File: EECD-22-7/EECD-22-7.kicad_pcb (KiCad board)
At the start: 2 copper layers, 55 parts, among them J1 Screw_Terminal_01x03, J2 Screw_Terminal_01x04, J3 Screw_Terminal_01x02, J4 Conn_ARM_JTAG_SWD_10, J5 Screw_Terminal_01x02, Q1 IRF6616, Q2 IRF6616, SW1 SW_Push, U1 4002B, U10 STM32F103CBUx, U7 LMR54406DBVR, U8 LMR54406DBVR, U9 LMR54406DBVR

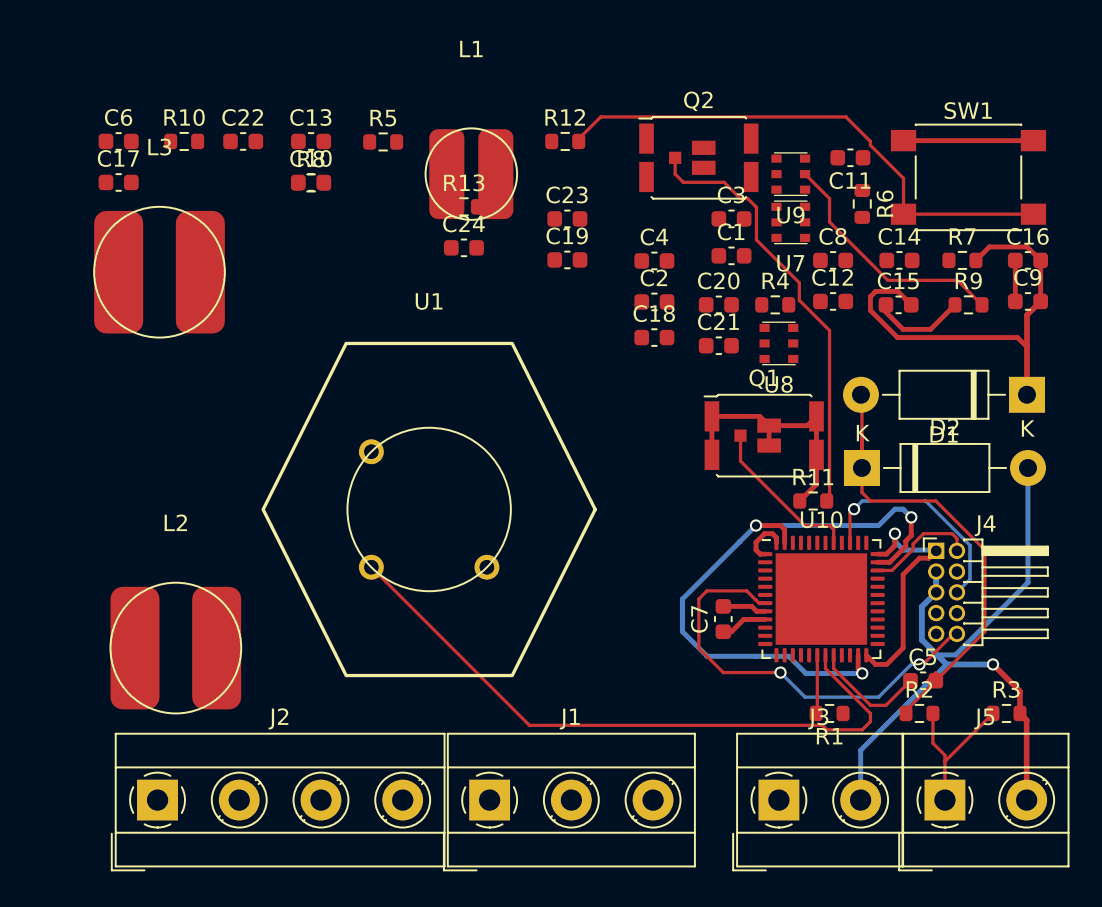
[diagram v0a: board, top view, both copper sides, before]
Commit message: Add files via upload
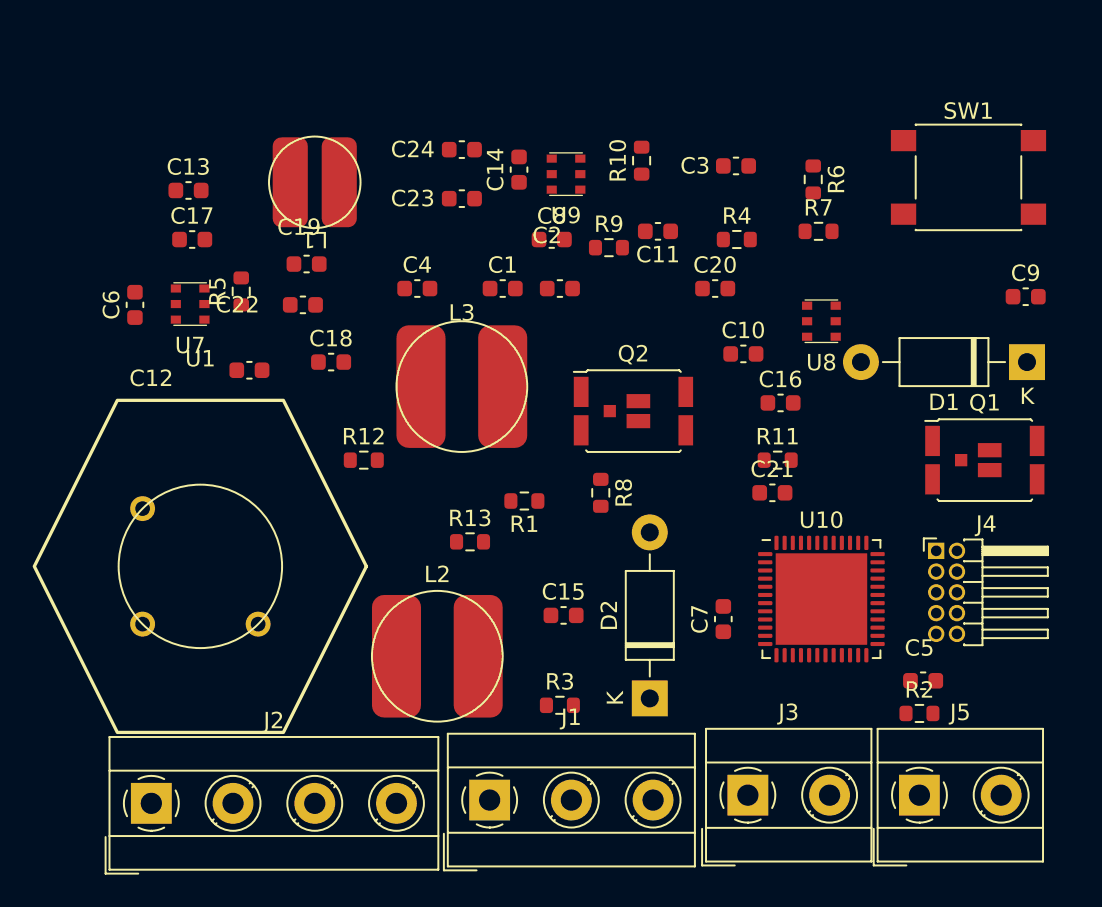
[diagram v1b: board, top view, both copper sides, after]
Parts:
- moved U7 37.1 mm to (116.4, 84.0)
- moved C12 36.0 mm to (120.0, 88.0)
- moved C10 28.5 mm to (150.2, 87.0)
- moved R10 28.0 mm to (144.0, 75.2), turned to 90 degrees
- moved C15 28.0 mm to (139.2, 103.0)
- moved R3 27.3 mm to (139.0, 108.5)
- moved R8 26.0 mm to (141.5, 95.5), turned to -90 degrees
- moved C14 23.9 mm to (136.5, 75.7), turned to 90 degrees
- moved R12 23.1 mm to (127.0, 93.5)
- moved R1 22.8 mm to (136.8, 96.0)
- moved R9 22.3 mm to (142.0, 80.5)
- moved R13 20.5 mm to (133.5, 98.5)
- moved C18 19.8 mm to (125.0, 87.5)
- moved L3 19.8 mm to (133.0, 89.0)
- moved D2 19.2 mm to (144.5, 108.1), turned to 90 degrees
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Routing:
- net GND12V: track 89.8 -> 0.00 mm, vias 1 -> 0
- net pres: track 40.1 -> 0.00 mm
- net 3.3V_GND: track 38.5 -> 0.00 mm, vias 3 -> 0
- net Net-(R12-Pad2): track 32.4 -> 0.00 mm
- net Net-(C5-Pad2): track 29.7 -> 0.00 mm
- net +3.3V: track 29.1 -> 0.00 mm, vias 1 -> 0
- net peri_power_2: track 26.7 -> 0.00 mm
- net RST: track 26.2 -> 0.00 mm, vias 2 -> 0
- net Net-(R10-Pad1): track 15.0 -> 0.00 mm
- net TDO: track 13.8 -> 0.00 mm, vias 1 -> 0
- net peri_power_1: track 9.81 -> 0.00 mm
- net Net-(BZ1-Pad1): track 9.76 -> 0.00 mm
- net acoustic: track 7.29 -> 0.00 mm
- net SWDIO: track 6.85 -> 0.00 mm
- net +5V: track 5.73 -> 0.00 mm
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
